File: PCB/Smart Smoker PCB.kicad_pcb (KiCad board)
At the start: 2 copper layers, 80 x 50 mm, 22 parts, among them J1 AC_IN, J2 Hopper, J3 Lid, U1 ESP32-WROOM-32UE_16MB, U2 DG409LEDY-T1-GE3, U3 MAX31855KASA

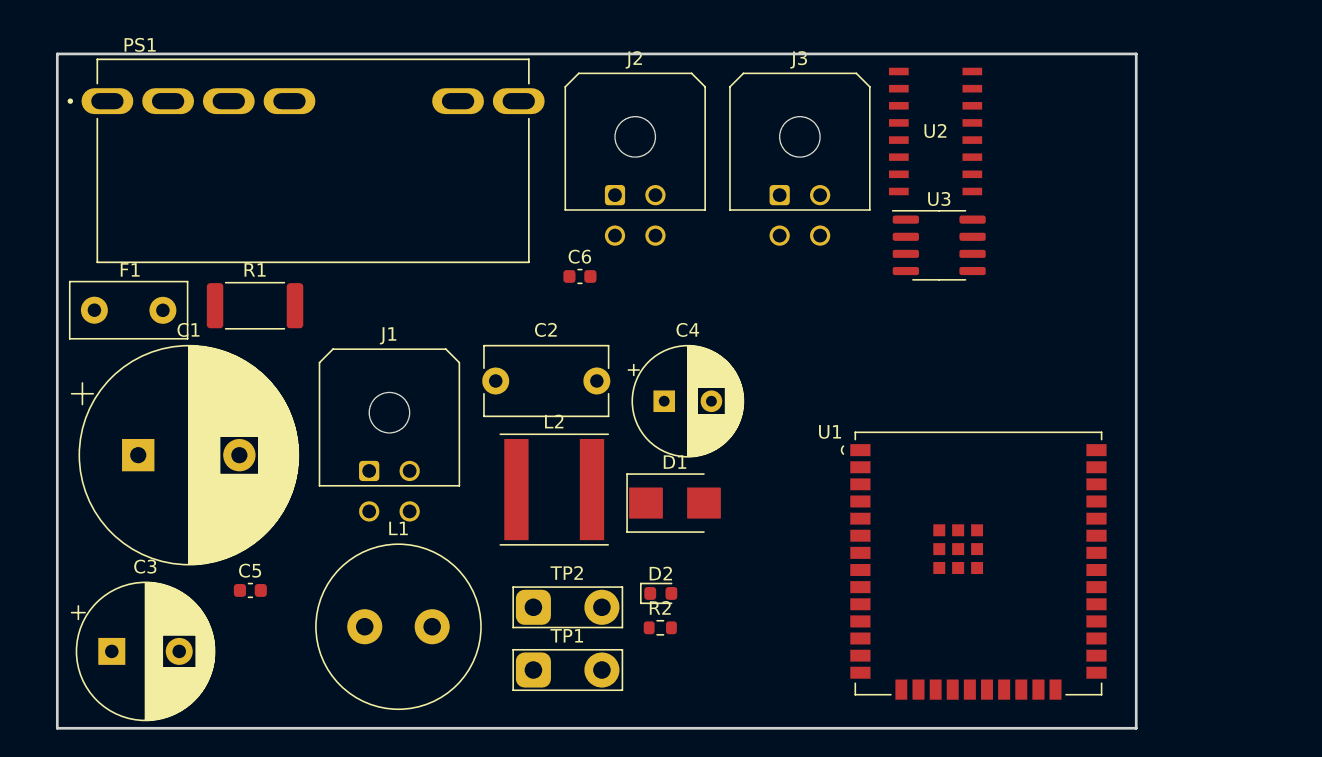
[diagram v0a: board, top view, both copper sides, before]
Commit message: PCB layout done
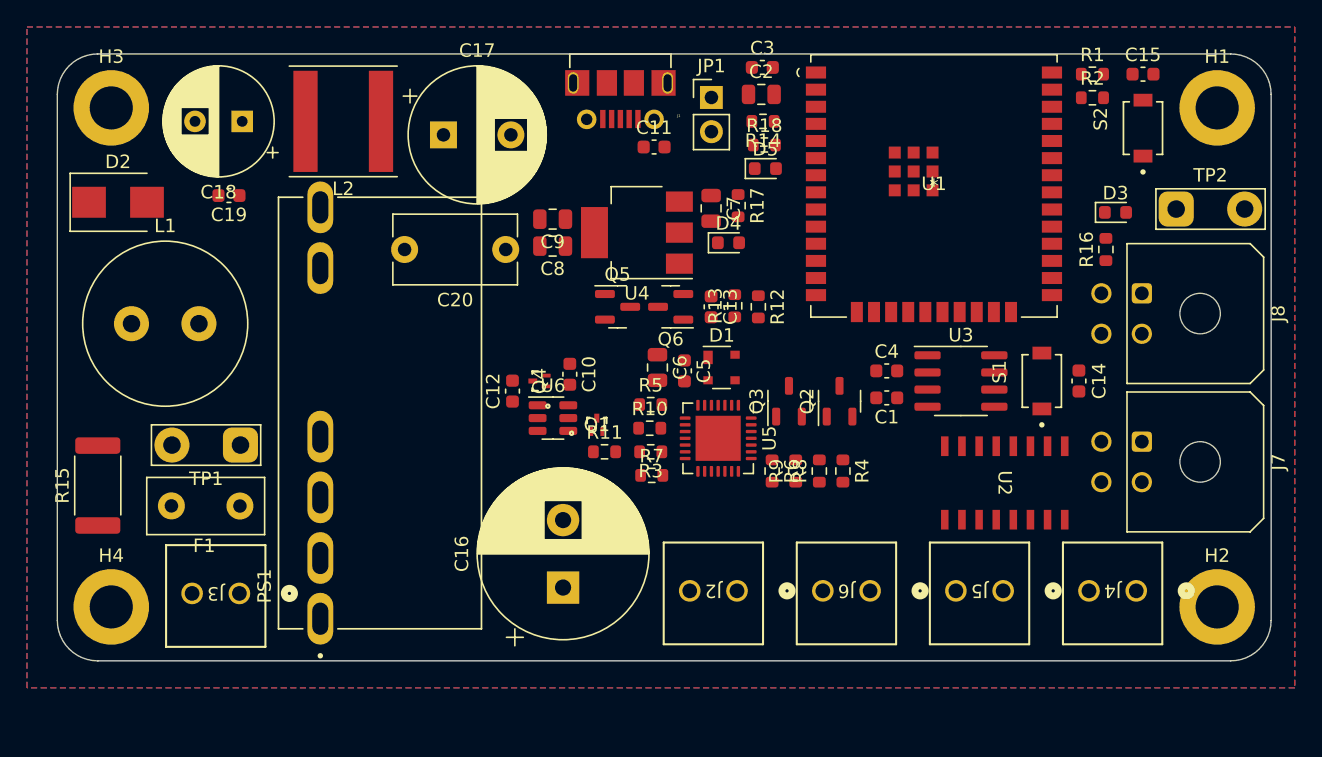
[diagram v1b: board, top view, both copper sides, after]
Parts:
- added C10: 1uF 25V X5R 0603, Capacitor_SMD:C_0603_1608Metric, F.Cu at (138.0, 123.8)
- added C11: 0.1uF 50V X7R 0603, Capacitor_SMD:C_0603_1608Metric, F.Cu at (144.2, 106.9)
- added C12: 0.1uF 50V X7R 0603, Capacitor_SMD:C_0603_1608Metric, F.Cu at (133.8, 125.0)
- added C13: 0.1uF 50V X7R 0603, Capacitor_SMD:C_0603_1608Metric, F.Cu at (148.5, 118.8)
- added C14: 0.1uF 50V X7R 0603, Capacitor_SMD:C_0603_1608Metric, F.Cu at (175.8, 124.2)
- added C15: 1uF 25V X5R 0603, Capacitor_SMD:C_0603_1608Metric, F.Cu at (180.5, 101.5)
- added C16: 22uF 450V 20%, Capacitor_THT:CP_Radial_D12.5mm_P5.00mm, F.Cu at (137.5, 139.6)
- added C17: 820uF 20% 16V, Capacitor_THT:CP_Radial_D10.0mm_P5.00mm, F.Cu at (128.6, 106.0)
- added C18: 150uF 20% 35V, Capacitor_THT:CP_Radial_D8.0mm_P3.50mm, F.Cu at (113.7, 105.0)
- added C19: 0.1uF 50V X7R 0603, Capacitor_SMD:C_0603_1608Metric, F.Cu at (112.7, 110.5)
- added C20: 1000pF 440VAC Y5P, Capacitor_THT:C_Disc_D9.0mm_W5.0mm_P7.50mm, F.Cu at (133.2, 114.5)
- added C7: 10uF 16V X5R 0805, Capacitor_SMD:C_0805_2012Metric, F.Cu at (148.5, 111.5)
- added C8: 10uF 16V X5R 0805, Capacitor_SMD:C_0805_2012Metric, F.Cu at (136.7, 114.2)
- added C9: 10uF 16V X5R 0805, Capacitor_SMD:C_0805_2012Metric, F.Cu at (136.7, 112.2)
- added D3: Y 2V 20mA, LED_SMD:LED_0603_1608Metric, F.Cu at (178.5, 111.8)
- added D4: Y/G 2.2V 20mA, LED_SMD:LED_0603_1608Metric, F.Cu at (149.8, 114.0)
- added D5: R 1.8V 2mA 0603, LED_SMD:LED_0603_1608Metric, F.Cu at (152.5, 108.5)
- added H1: MountingHole, MountingHole:MountingHole_3.2mm_M3_DIN965_Pad, F.Cu at (186.0, 104.0)
- added H2: MountingHole, MountingHole:MountingHole_3.2mm_M3_DIN965_Pad, F.Cu at (186.0, 141.0)
- added H3: MountingHole, MountingHole:MountingHole_3.2mm_M3_DIN965_Pad, F.Cu at (104.0, 104.0)
- added H4: MountingHole, MountingHole:MountingHole_3.2mm_M3_DIN965_Pad, F.Cu at (104.0, 141.0)
- added J4: 393570002, Customs Smoker:CONN_393570002_MOL, F.Cu at (180.0, 139.8)
- added J5: 393570002, Customs Smoker:CONN_393570002_MOL, F.Cu at (170.1, 139.8)
- added J6: 393570002, Customs Smoker:CONN_393570002_MOL, F.Cu at (160.3, 139.8)
- added J7: Hopper, Connector_Molex:Molex_Micro-Fit_3.0_43045-0400_2x02_P3.00mm_Horizontal, F.Cu at (180.4, 128.8)
- added J8: Lid, Connector_Molex:Molex_Micro-Fit_3.0_43045-0400_2x02_P3.00mm_Horizontal, F.Cu at (180.4, 117.8)
- added JP1: Jumper_2_Open, Connector_PinHeader_2.54mm:PinHeader_1x02_P2.54mm_Vertical, F.Cu at (148.5, 103.2)
- added Q1: Q_PMOS_GSD, Customs Smoker:VESM_TOS, F.Cu at (140.0, 127.5)
- added Q2: 25V 1.5A Trans, Package_TO_SOT_SMD:SOT-23-3, F.Cu at (158.0, 125.8)
- added Q3: 25V 1.5A Trans, Package_TO_SOT_SMD:SOT-23-3, F.Cu at (154.2, 125.8)
- added Q4: Q_PMOS_GSD, Customs Smoker:VESM_TOS, F.Cu at (135.8, 124.2)
- added Q5: 2N7002T-7-F, Package_TO_SOT_SMD:SOT-23, F.Cu at (141.5, 118.8)
- added Q6: 2N7002T-7-F, Package_TO_SOT_SMD:SOT-23, F.Cu at (145.5, 118.8)
- added R10: 47.5kOhm 1% 0603, Resistor_SMD:R_0603_1608Metric, F.Cu at (143.9, 127.8)
- added R11: 470Ohm 5% 0603, Resistor_SMD:R_0603_1608Metric, F.Cu at (140.6, 129.5)
- added R12: 1kOhm 1% 0603, Resistor_SMD:R_0603_1608Metric, F.Cu at (152.0, 118.8)
- added R13: 10K 1% 0603, Resistor_SMD:R_0603_1608Metric, F.Cu at (150.2, 118.7)
- added R14: 10K 1% 0603, Resistor_SMD:R_0603_1608Metric, F.Cu at (152.3, 105.0)
- added R15: 6.8Ohm 3W 5% 2512, Resistor_SMD:R_2512_6332Metric, F.Cu at (103.0, 132.0)
- added R16: 470Ohm 1% 0603, Resistor_SMD:R_0603_1608Metric, F.Cu at (177.8, 114.5)
- added R17: 140Ohm 1% 0603, Resistor_SMD:R_0603_1608Metric, F.Cu at (150.5, 111.2)
- added R18: 750Ohm 1% 0603, Resistor_SMD:R_0603_1608Metric, F.Cu at (152.4, 106.8)
- added R3: 1kOhm 1% 0603, Resistor_SMD:R_0603_1608Metric, F.Cu at (144.0, 129.5)
- added R4: 10K 1% 0603, Resistor_SMD:R_0603_1608Metric, F.Cu at (158.2, 130.9)
- added R5: 22.1kOhm 1% 0603, Resistor_SMD:R_0603_1608Metric, F.Cu at (144.0, 126.0)
- added R6: 10K 1% 0603, Resistor_SMD:R_0603_1608Metric, F.Cu at (153.0, 130.9)
- added R7: 10K 1% 0603, Resistor_SMD:R_0603_1608Metric, F.Cu at (144.1, 131.2)
- added R8: 0Ohm 0603, Resistor_SMD:R_0603_1608Metric, F.Cu at (156.5, 130.9)
- added R9: 0Ohm 0603, Resistor_SMD:R_0603_1608Metric, F.Cu at (154.8, 130.9)
- added S1: TL1015AF160QG, Customs Smoker:SW_TL1015AF160QG, F.Cu at (173.0, 124.2)
- added S2: TL1015AF160QG, Customs Smoker:SW_TL1015AF160QG, F.Cu at (180.5, 105.5)
- added U4: AMS1117-3.3, Package_TO_SOT_SMD:SOT-223-3_TabPin2, F.Cu at (143.0, 113.2)
- added U5: CP2102N-Axx-xQFN28, Package_DFN_QFN:QFN-28-1EP_5x5mm_P0.5mm_EP3.35x3.35mm, F.Cu at (149.0, 128.5)
- added U6: LTC4412xS6, Package_TO_SOT_SMD:TSOT-23-6, F.Cu at (136.8, 127.0)
- C1: value 22uF 450V 20% -> 0.1uF 50V X7R 0603; footprint Capacitor_THT:CP_Radial_D16.0mm_P7.50mm -> Capacitor_SMD:C_0603_1608Metric
- C2: value 1000pF 440VAC Y5P -> 22uF 10V X5R 0805; footprint Capacitor_THT:C_Disc_D9.0mm_W5.0mm_P7.50mm -> Capacitor_SMD:C_0805_2012Metric
- C3: value 820uF 20% 16V -> 0.1uF 50V X7R 0603; footprint Capacitor_THT:CP_Radial_D10.0mm_P5.00mm -> Capacitor_SMD:C_0603_1608Metric
- C4: value 150uF 20% 35V -> 0.01uF 50V X7R 0603; footprint Capacitor_THT:CP_Radial_D8.0mm_P3.50mm -> Capacitor_SMD:C_0603_1608Metric
- C6: value 0.1uF 50V X7R 0603 -> 4.7uF 25V X5R 0805; footprint Capacitor_SMD:C_0603_1608Metric -> Capacitor_SMD:C_0805_2012Metric
- D1: value TVS DIODE 7VWM 12VC SMB -> SP0503BAHT; footprint Diode_SMD:D_SMB -> Package_TO_SOT_SMD:SOT-143
- D2: value LED -> TVS DIODE 7VWM 12VC SMB; footprint LED_SMD:LED_0603_1608Metric -> Diode_SMD:D_SMB
- F1: value 300V 1A SlowBlow -> 300V 2A SlowBlow
- J1: value AC_IN -> 105017-0001; footprint Connector_Molex:Molex_Micro-Fit_3.0_43045-0400_2x02_P3.00mm_Horizontal -> Customs Smoker:MOLEX_105017-0001
- J2: value Hopper -> 393570002; footprint Connector_Molex:Molex_Micro-Fit_3.0_43045-0400_2x02_P3.00mm_Horizontal -> Customs Smoker:CONN_393570002_MOL
- J3: value Lid -> 393570002; footprint Connector_Molex:Molex_Micro-Fit_3.0_43045-0400_2x02_P3.00mm_Horizontal -> Customs Smoker:CONN_393570002_MOL
- R1: value 6.8Ohm 3W 5% 2512 -> 1kOhm 1% 0603; footprint Resistor_SMD:R_2512_6332Metric -> Resistor_SMD:R_0603_1608Metric
- R2: value R_US -> 1kOhm 1% 0603
- moved C3 64.8 mm to (152.3, 101.0)
- moved R1 64.4 mm to (176.8, 101.5)
- moved TP2 56.1 mm to (183.0, 111.5)
- moved C1 55.7 mm to (161.5, 125.5), turned to 180 degrees
- moved R2 50.7 mm to (176.8, 103.2)
- moved J3 49.8 mm to (113.5, 140.0), turned to 180 degrees
- moved D2 49.6 mm to (104.5, 111.0)
- moved C5 36.1 mm to (146.5, 123.5), turned to -90 degrees
- moved J1 34.3 mm to (141.8, 102.2), turned to 180 degrees
- moved L2 31.5 mm to (121.2, 105.0), turned to 180 degrees
- moved J2 30.7 mm to (150.4, 139.8), turned to 180 degrees
- moved C2 29.0 mm to (152.2, 103.0)
- moved L1 28.4 mm to (105.5, 120.0)
- moved U1 28.2 mm to (165.0, 109.8)
- moved TP1 27.4 mm to (113.6, 129.0), turned to 180 degrees
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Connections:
- C1 pad 1: Net-(PS1-Pad3) -> +3.3V
- C1 pad 2: Net-(PS1-Pad4) -> GND
- C2 pad 1: Net-(PS1-Pad4) -> GND
- C2 pad 2: GND -> +3.3V
- C3 pad 1: Net-(L2-Pad1) -> GND
- C3 pad 2: GND -> +3.3V
- C4 pad 1: +3.3V -> /MUX_OUT_+
- C4 pad 2: GND -> /MUX_OUT_-
- C5 pad 1: +3.3V -> GND
- C5 pad 2: GND -> +3.3V
- C6 pad 1: +3.3V -> GND
- C6 pad 2: GND -> +3.3V
- D1 pad 2: +3.3V -> /USB_DP
- D2 pad 2: Net-(D2-Pad2) -> +3.3VA
- F1 pad 2: Net-(R1-Pad1) -> Net-(F1-Pad2)
- J1 pad 1: /AC_L -> +5V
- J1 pad 2: /AC_N -> /USB_DN
- J1 pad 3: unconnected-(J1-Pad3) -> /USB_DP
- J2 pad 1: /SDA -> /Probe4+
- J2 pad 2: GND -> /Probe4-
- J3 pad 1: /SDA -> /AC_L
- J3 pad 2: GND -> /AC_N
- L2 pad 1: Net-(L2-Pad1) -> Net-(C17-Pad1)
- L2 pad 2: +3.3V -> +3.3VA
- PS1 pad 3: Net-(PS1-Pad3) -> Net-(C16-Pad1)
- PS1 pad 4: Net-(PS1-Pad4) -> Net-(C20-Pad1)
- PS1 pad 6: Net-(L2-Pad1) -> Net-(C17-Pad1)
- R1 pad 1: Net-(R1-Pad1) -> /I2C_SCL
- R1 pad 2: Net-(L1-Pad1) -> +3.3V
- R2 pad 1: +3.3V -> /I2C_SDA
- R2 pad 2: Net-(D2-Pad2) -> +3.3V
- U1 pad 1: unconnected-(U1-Pad1) -> GND
- U1 pad 10: unconnected-(U1-Pad10) -> /IO25
- U1 pad 11: unconnected-(U1-Pad11) -> /IO26
- U1 pad 12: unconnected-(U1-Pad12) -> /IO27
- U1 pad 13: unconnected-(U1-Pad13) -> /IO14
- U1 pad 14: unconnected-(U1-Pad14) -> /IO12
- U1 pad 15: unconnected-(U1-Pad15) -> GND
- U1 pad 16: unconnected-(U1-Pad16) -> /IO13
- U1 pad 2: unconnected-(U1-Pad2) -> +3.3V
- U1 pad 23: unconnected-(U1-Pad23) -> /IO15
- U1 pad 24: unconnected-(U1-Pad24) -> /IO2
- U1 pad 25: unconnected-(U1-Pad25) -> /IO0
- U1 pad 26: unconnected-(U1-Pad26) -> /IO4
- U1 pad 27: unconnected-(U1-Pad27) -> /IO16
- U1 pad 28: unconnected-(U1-Pad28) -> /IO17
- U1 pad 29: unconnected-(U1-Pad29) -> /SPI_CS
- U1 pad 3: unconnected-(U1-Pad3) -> /EN
- U1 pad 30: unconnected-(U1-Pad30) -> /SPI_SCK
- U1 pad 31: unconnected-(U1-Pad31) -> /SPI_MISO
- U1 pad 33: unconnected-(U1-Pad33) -> /I2C_SDA
- U1 pad 34: unconnected-(U1-Pad34) -> /RXD0
- U1 pad 35: unconnected-(U1-Pad35) -> /TXD0
- U1 pad 36: unconnected-(U1-Pad36) -> /I2C_SCL
- U1 pad 37: unconnected-(U1-Pad37) -> /IO23
- U1 pad 38: unconnected-(U1-Pad38) -> GND
- U1 pad 39: unconnected-(U1-Pad39) -> GND
- U1 pad 4: unconnected-(U1-Pad4) -> /I36
- U1 pad 40: unconnected-(U1-Pad40) -> GND
- U1 pad 41: unconnected-(U1-Pad41) -> GND
- U1 pad 42: unconnected-(U1-Pad42) -> GND
- U1 pad 43: unconnected-(U1-Pad43) -> GND
- U1 pad 44: unconnected-(U1-Pad44) -> GND
- U1 pad 45: unconnected-(U1-Pad45) -> GND
- U1 pad 46: unconnected-(U1-Pad46) -> GND
- U1 pad 47: unconnected-(U1-Pad47) -> GND
- U1 pad 5: unconnected-(U1-Pad5) -> /I39
- U1 pad 6: unconnected-(U1-Pad6) -> /I34
- U1 pad 7: unconnected-(U1-Pad7) -> /I35
- U1 pad 8: unconnected-(U1-Pad8) -> /IO32
- U1 pad 9: unconnected-(U1-Pad9) -> /IO33
- U2 pad 1: unconnected-(U2-Pad1) -> /IO2
- U2 pad 10: unconnected-(U2-Pad10) -> /Probe4+
- U2 pad 11: unconnected-(U2-Pad11) -> /Probe3+
- U2 pad 12: unconnected-(U2-Pad12) -> /Probe2+
- U2 pad 13: unconnected-(U2-Pad13) -> /Probe1+
- U2 pad 14: unconnected-(U2-Pad14) -> +3.3V
- U2 pad 15: unconnected-(U2-Pad15) -> GND
- U2 pad 16: unconnected-(U2-Pad16) -> /IO15
- U2 pad 2: unconnected-(U2-Pad2) -> +3.3V
- U2 pad 3: unconnected-(U2-Pad3) -> GND
- U2 pad 4: unconnected-(U2-Pad4) -> /Probe1-
- U2 pad 5: unconnected-(U2-Pad5) -> /Probe2-
- U2 pad 6: unconnected-(U2-Pad6) -> /Probe3-
- U2 pad 7: unconnected-(U2-Pad7) -> /Probe4-
- U2 pad 8: unconnected-(U2-Pad8) -> /MUX_OUT_-
- U2 pad 9: unconnected-(U2-Pad9) -> /MUX_OUT_+
- U3 pad 2: unconnected-(U3-Pad2) -> /MUX_OUT_-
- U3 pad 3: unconnected-(U3-Pad3) -> /MUX_OUT_+
- U3 pad 5: unconnected-(U3-Pad5) -> /SPI_SCK
- U3 pad 6: unconnected-(U3-Pad6) -> /SPI_CS
- U3 pad 7: unconnected-(U3-Pad7) -> /SPI_MISO
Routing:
- added copper zone on In2.Cu, net +3.3V
- added copper zone on B.Cu, net GND
- added copper zone on F.Cu, net GND
- added copper zone on In1.Cu, net GND
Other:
- board size 80 x 50 mm -> 90 x 45 mm
- copper layers 2 -> 4
